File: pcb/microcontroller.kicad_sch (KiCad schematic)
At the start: 24 parts, among them J1 TC2030, J3 TC2030, U3 74HCT541, U4 STM32F103C8T6, U5 SN65HVD230, Y1 8MHz

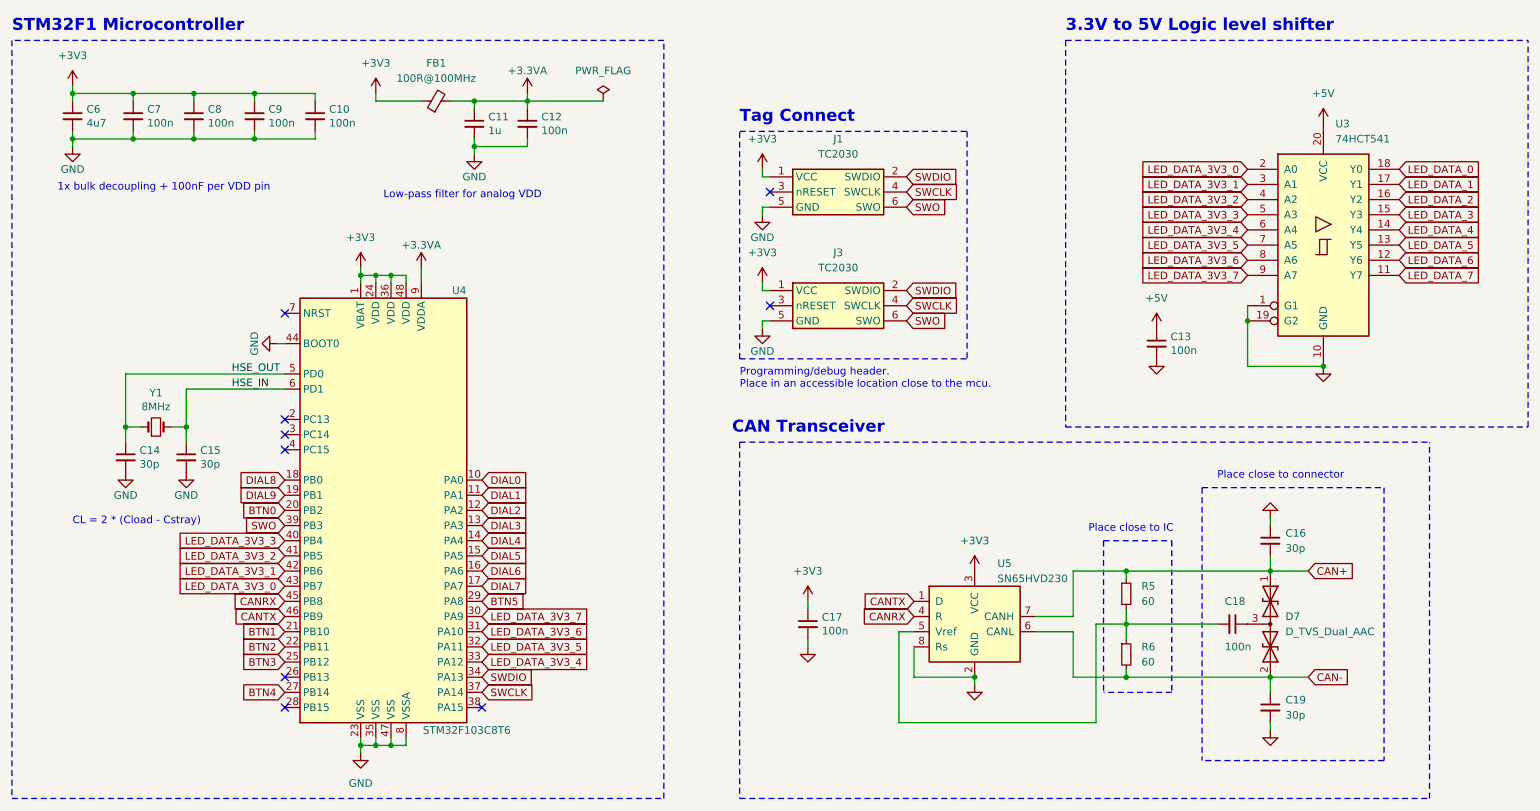
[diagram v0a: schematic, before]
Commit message: added br24 changes
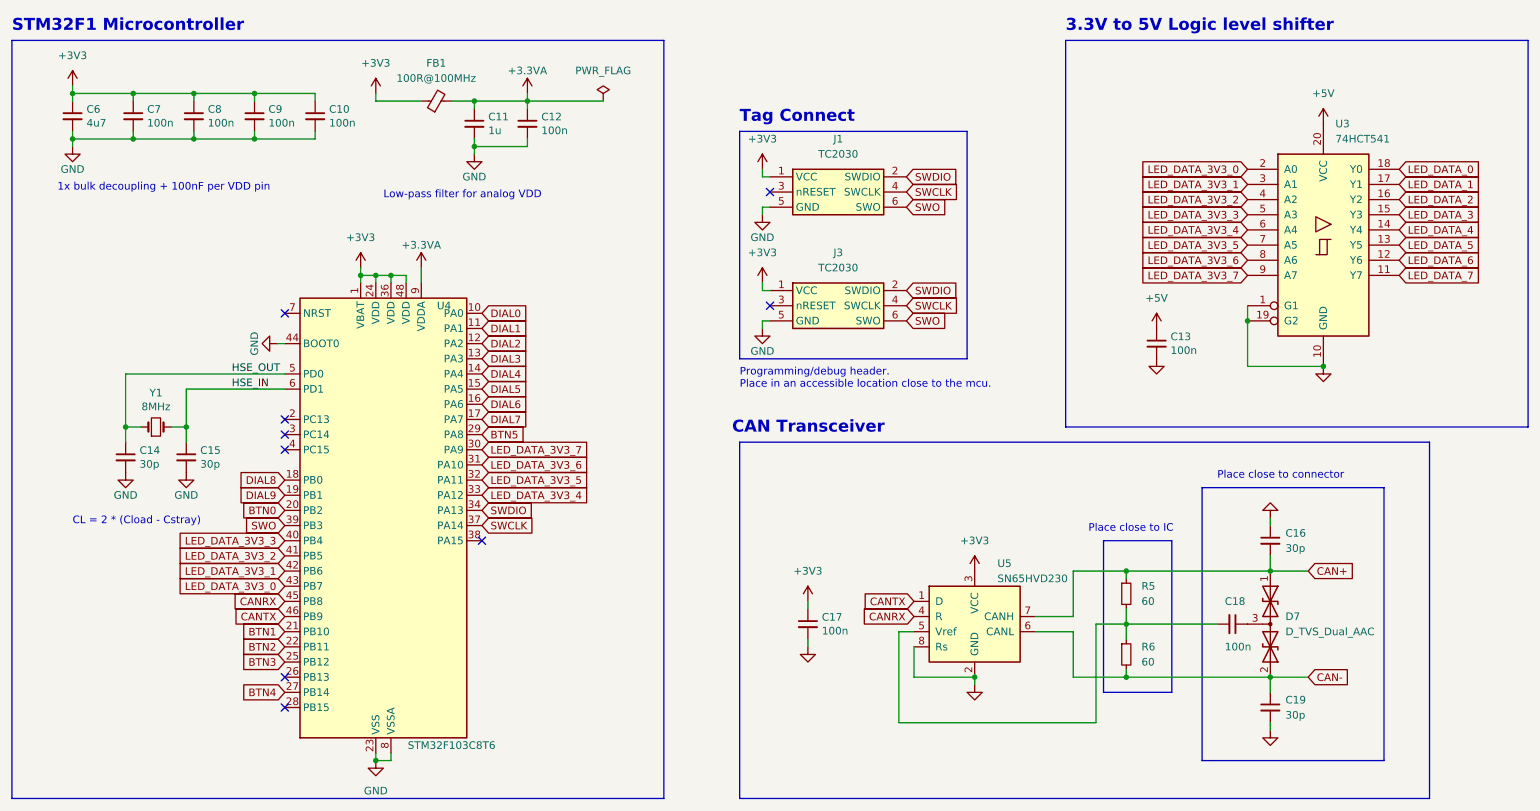
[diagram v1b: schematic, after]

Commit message: LED Footprints fixed
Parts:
- R5, R6: LCSC C441730 -> C844855
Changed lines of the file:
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@@
 			)
 		)
-		(property "LCSC" "C441730"
+		(property "LCSC" "C844855"
 			(at 212.09 119.38 0)
 			(effects
@@
 			)
 		)
-		(property "LCSC" "C441730"
+		(property "LCSC" "C844855"
 			(at 212.09 129.54 0)
 			(effects
